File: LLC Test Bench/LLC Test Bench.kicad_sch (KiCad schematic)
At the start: 26 parts, among them J1 +HV, J2 -HV, J3 +LV, J4 -LV, Q1 NMOS, Q2 NMOS, Q3 NMOS, Q4 NMOS, T1 Transformer_SP_2S, U3 Optocoupler, U4 TL431D

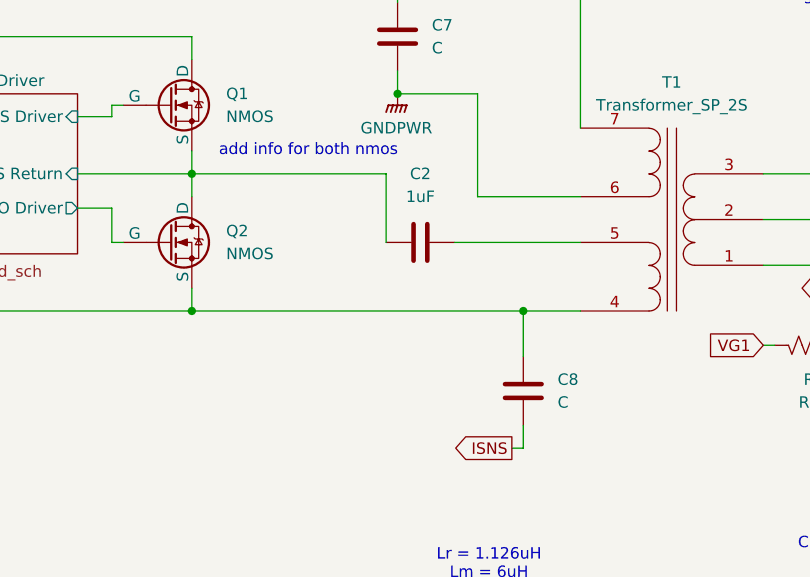
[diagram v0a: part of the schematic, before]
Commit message: Changes to ISNS
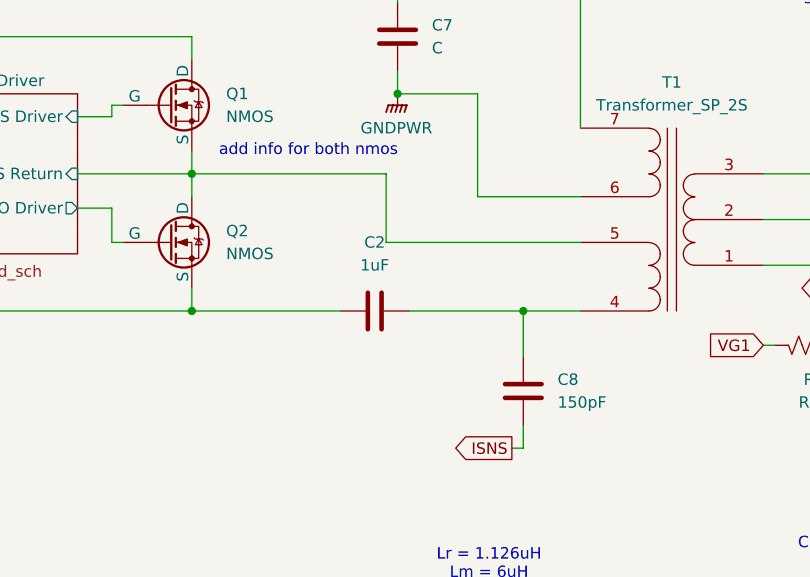
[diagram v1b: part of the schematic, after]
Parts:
- C8: value C -> 150pF
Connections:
- net GNDPWR: now also C2.1; no longer C8.1, T1.4 (OUT1A)
- net LLC Controller/Gate Driver/HS Return: now also T1.5 (OUT1B); no longer C2.1
- net at C2.2: now also C8.1, T1.4 (OUT1A); no longer T1.5 (OUT1B)
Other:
- moved on the sheet: C2
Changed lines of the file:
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@@
 	(wire
 		(pts
+			(xy 165.1 146.05) (xy 186.69 146.05)
+		)
+		(stroke
+			(width 0)
+			(type default)
+		)
+	)
+	(wire
+		(pts
 			(xy 242.57 157.48) (xy 243.84 157.48)
 		)
@@
 	(wire
 		(pts
-			(xy 143.51 153.67) (xy 180.34 153.67)
+			(xy 143.51 153.67) (xy 160.02 153.67)
 		)
 		(stroke
@@
 	(wire
 		(pts
-			(xy 172.72 146.05) (xy 186.69 146.05)
-		)
-		(stroke
-			(width 0)
-			(type default)
-		)
-	)
-	(wire
-		(pts
 			(xy 267.97 191.77) (xy 267.97 196.85)
 		)
@@
 	(wire
 		(pts
+			(xy 167.64 153.67) (xy 180.34 153.67)
+		)
+		(stroke
+			(width 0)
+			(type default)
+		)
+	)
+	(wire
+		(pts
 			(xy 262.89 191.77) (xy 267.97 191.77)
 		)
@@
 			)
 		)
-		(property "Value" "C"
+		(property "Value" "150pF"
 			(at 184.15 163.8299 0)
 			(effects
@@
 	(symbol
 		(lib_id "Device:C")
-		(at 168.91 146.05 90)
+		(at 163.83 153.67 90)
 		(unit 1)
 		(exclude_from_sim no)
@@
 		(fields_autoplaced yes)
 		(property "Reference" "C2"
-			(at 168.91 138.43 90)
+			(at 163.83 146.05 90)
 			(effects
 				(font
@@
 		)
 		(property "Value" "1uF"
-			(at 168.91 140.97 90)
+			(at 163.83 148.59 90)
 			(effects
 				(font
@@
 		)
 		(property "Footprint" ""
-			(at 172.72 145.0848 0)
+			(at 167.64 152.7048 0)
 			(effects
 				(font
@@
 		)
 		(property "Datasheet" "~"
-			(at 168.91 146.05 0)
+			(at 163.83 153.67 0)
 			(effects
 				(font
@@
 		)
 		(property "Description" "Unpolarized capacitor"
-			(at 168.91 146.05 0)
+			(at 163.83 153.67 0)
 			(effects
 				(font
